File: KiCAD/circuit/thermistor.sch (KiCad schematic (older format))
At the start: 24 parts, among them J1 To USB-UART converter, J10 Jumper, J11 Jumper, J12 Jumper, J13 Jumper, J14 Jumper, J15 Jumper, J16 Jumper, J2 Pin header, J3 Pin header, J4 2x4 pin header, J5 Jumper, J6 Jumper, J7 Jumper, J8 Jumper, J9 Jumper, U1 PIC16f1825-I/P

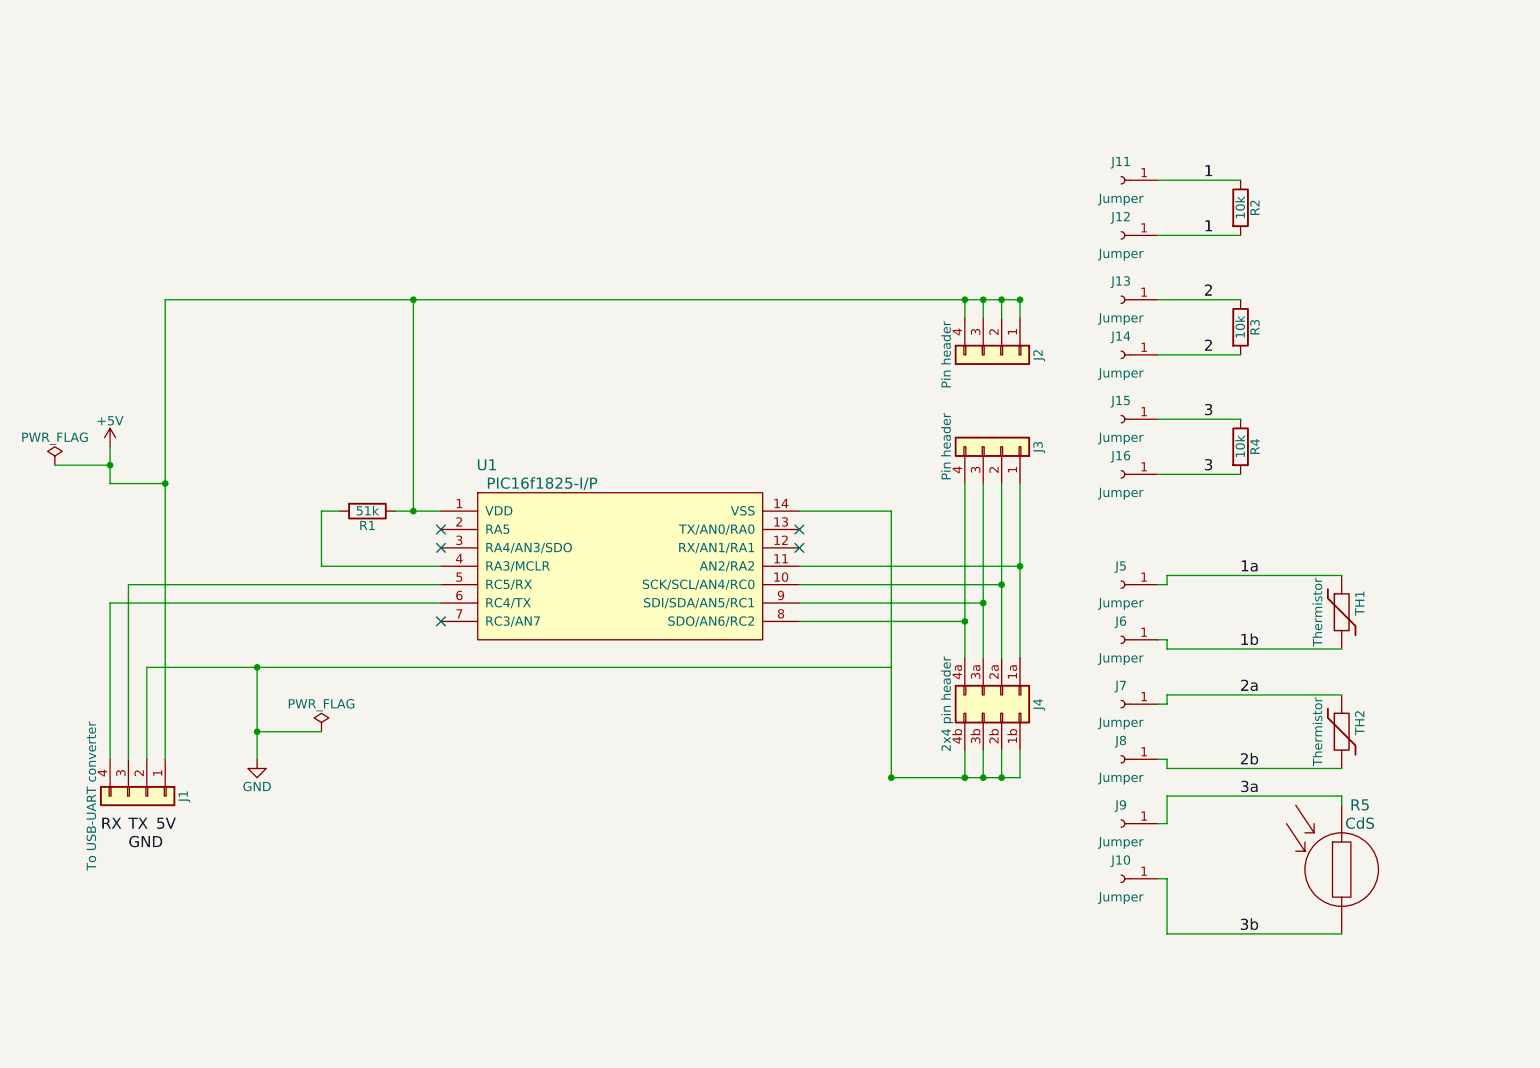
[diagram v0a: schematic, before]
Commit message: circuit update
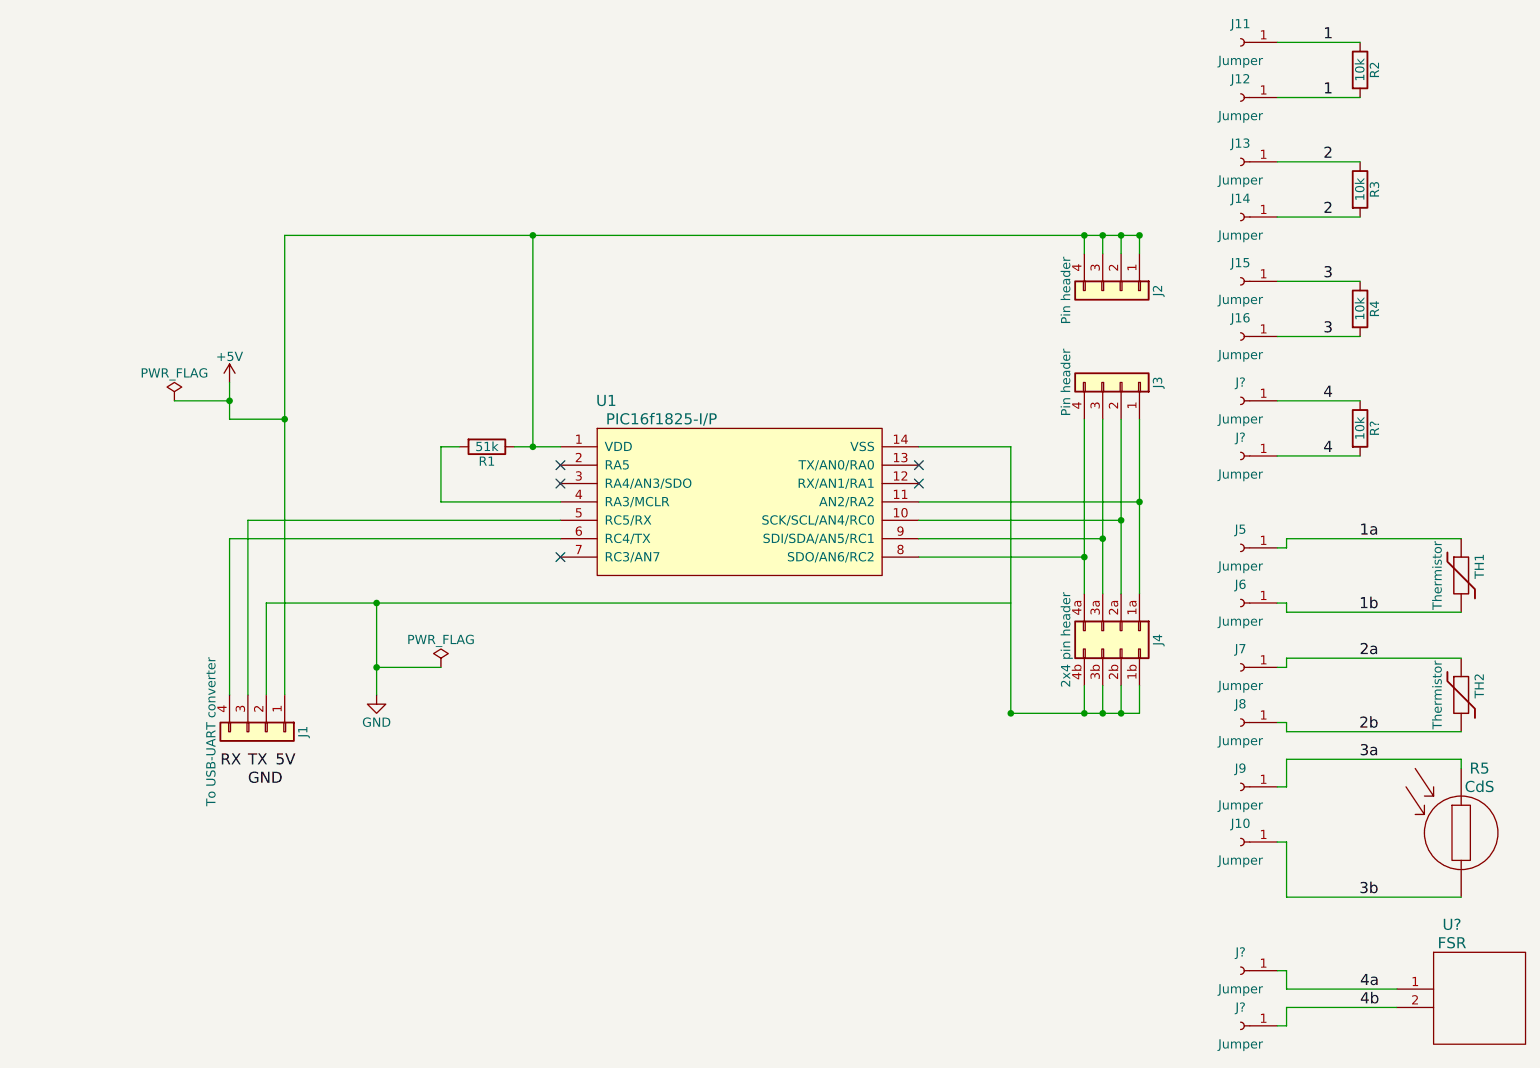
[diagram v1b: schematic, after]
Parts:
- added J? (x4): Jumper, symbol Conn_01x01_Female
- added R?: 10k, symbol R
- added U?: FSR, symbol FSR
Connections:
- new net 4: J?.1 (Pin_1), J?.1 (Pin_1), R?.1, R?.2
- new net 4a: J?.1 (Pin_1), U?.1
- new net 4b: J?.1 (Pin_1), U?.2
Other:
- moved on the sheet: J1, J10, J11, J12, J13, J14, J15, J16, J2, J3, J4, J5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
